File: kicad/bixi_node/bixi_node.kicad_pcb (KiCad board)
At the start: 2 copper layers, 48.3 x 16.5 mm, 8 parts, among them J1 RJ45, P1 CONN_01X03, U1 SP3485CN

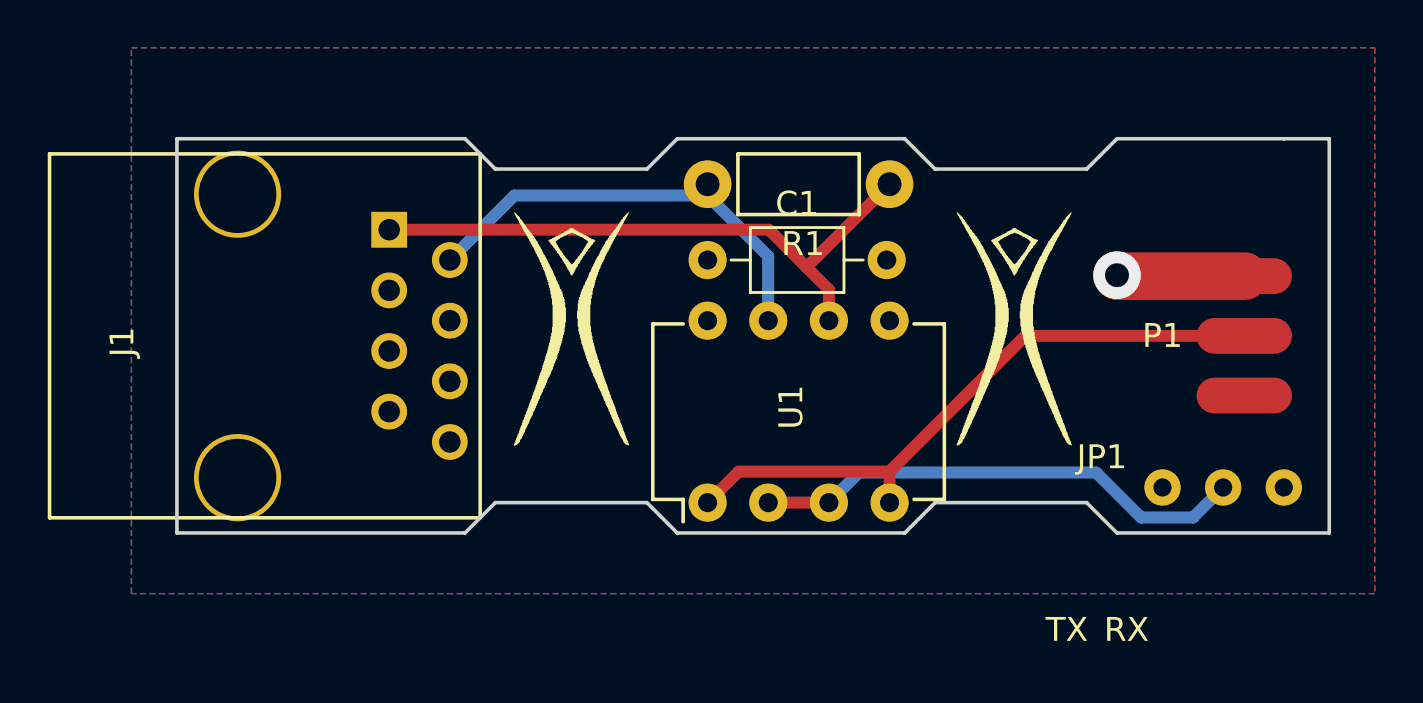
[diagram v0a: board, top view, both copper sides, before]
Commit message: fixes to boards, node still in progress
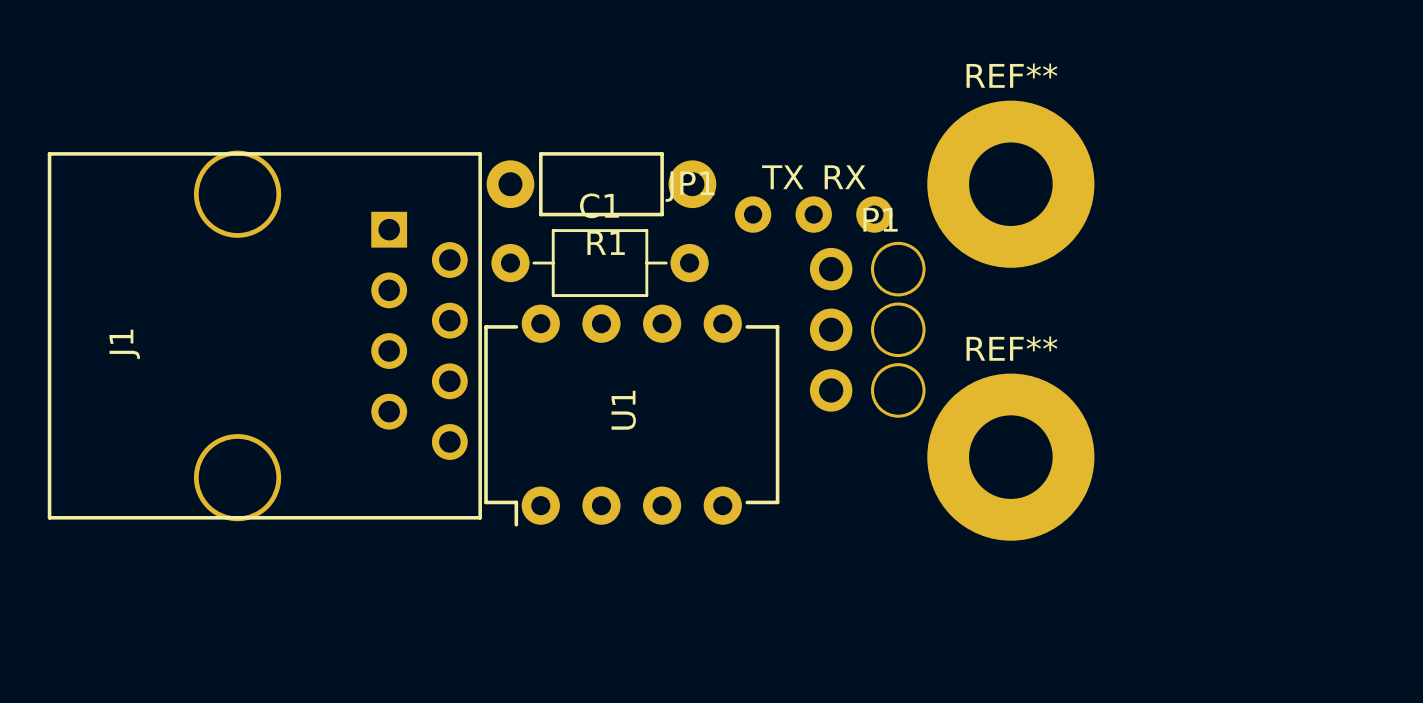
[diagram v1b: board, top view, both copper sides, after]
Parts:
- removed burner-logo1, burner-logo2: , logos:burner-logo-fs
- added REF**: MountingHole_3.5mm_Pad, Mounting_Holes:MountingHole_3.5mm_Pad, F.Cu at (128.9, 85.1)
- added REF**: MountingHole_3.5mm_Pad, Mounting_Holes:MountingHole_3.5mm_Pad, F.Cu at (128.9, 96.5)
- P1: footprint custom:PAD_3X_OVAL_WS2812B -> custom:3-wire-hole-with-relief
- moved JP1 20.6 mm to (120.7, 86.4)
- moved P1 15.2 mm to (123.2, 91.2), turned to 0 degrees
- moved C1 8.26 mm to (108.0, 88.4)
- moved R1 8.25 mm to (108.0, 85.1)
- moved U1 6.99 mm to (109.2, 98.6)
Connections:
- P1 pad 1: VCC -> GND
- P1 pad 3: GND -> Net-(P1-Pad3)
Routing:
- net /DATA: track 26.7 -> 0.00 mm
- net /DATA_DIFF_A: track 25.7 -> 0.00 mm
- net /MODE: track 20.9 -> 0.00 mm
- net /DATA_DIFF_B: track 18.7 -> 0.00 mm
- net GND: track 5.35 -> 0.00 mm, vias 1 -> 0
- removed copper zone on B.Cu, net GND
- removed copper zone on F.Cu, net VCC
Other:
- board outline removed

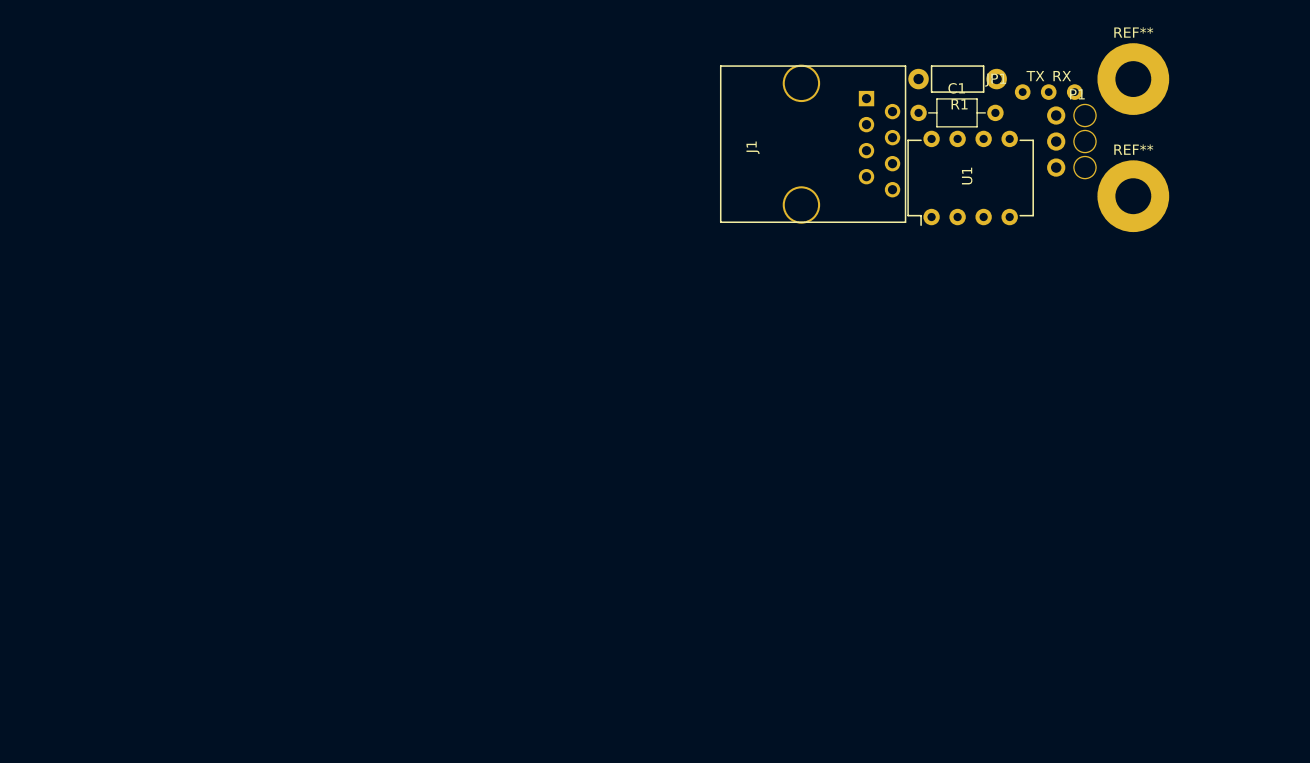
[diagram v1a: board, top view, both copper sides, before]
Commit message: node work for keystone box
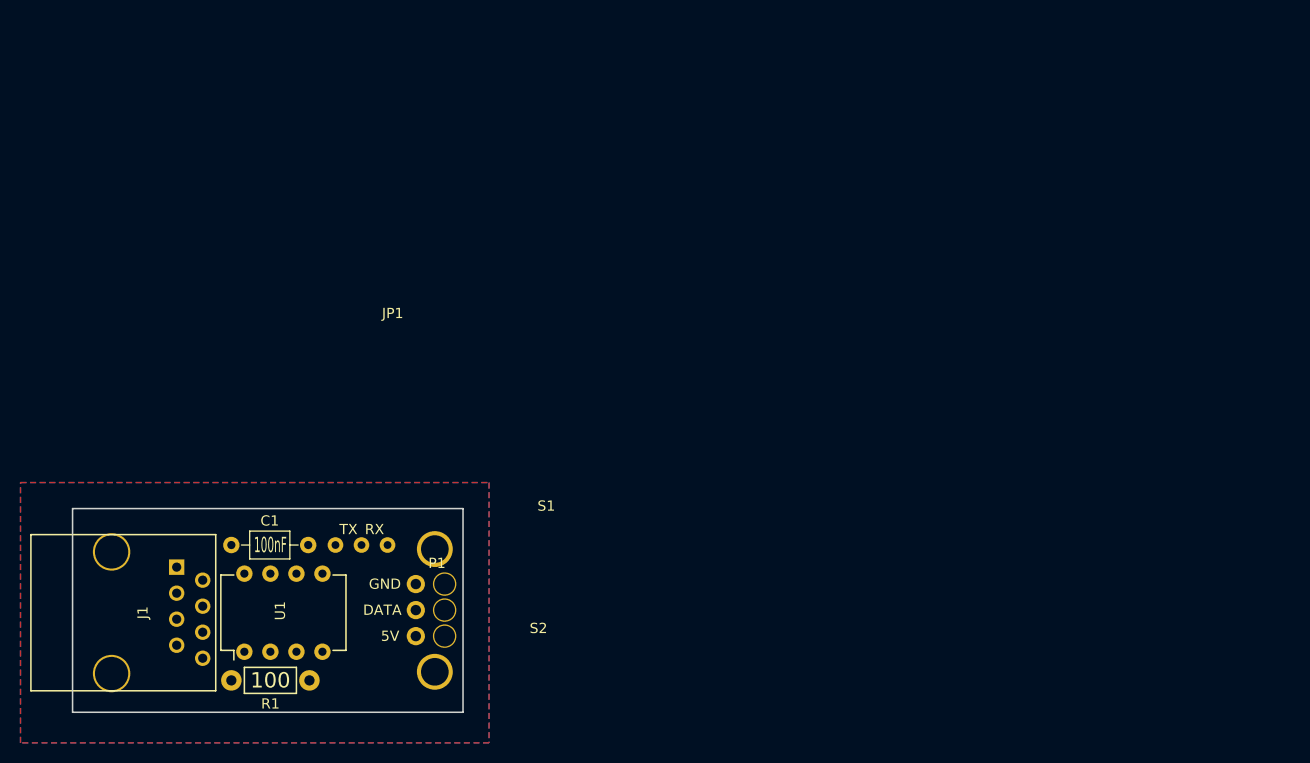
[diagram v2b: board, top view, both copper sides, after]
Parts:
- removed REF** (x2): MountingHole_3.5mm_Pad, Mounting_Holes:MountingHole_3.5mm_Pad
- added S1: MountingHole_2.7mm_Pad, Mounting_Holes:MountingHole_2.7mm_Pad, F.Cu at (60.8, 130.9)
- added S2: MountingHole_2.7mm_Pad, Mounting_Holes:MountingHole_2.7mm_Pad, F.Cu at (60.8, 142.9)
- moved R1 89.1 mm to (40.9, 143.8)
- moved J1 81.4 mm to (29.2, 137.2)
- moved JP1 80.3 mm to (53.6, 130.6)
- moved U1 79.3 mm to (42.2, 141.0)
- moved C1 79.2 mm to (40.9, 130.6)
- moved P1 77.4 mm to (60.7, 136.9)
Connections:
- P1 pad 3: Net-(P1-Pad3) -> VCC
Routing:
- added copper zone on B.Cu, net GND
- added copper zone on F.Cu, net VCC
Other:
- board outline added: 38.1 x 19.9 mm
- net class Default: trace_width 2 -> 0.4; via_dia 2 -> 0.4; via_drill 1 -> 0.3
- board text added: "100"
- board text added: "100nF"
- board text added: "5V"
- board text added: "DATA"
- board text added: "GND"
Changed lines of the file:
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@@
 (kicad_pcb (version 4) (host pcbnew 4.0.6)
   (general
-    (links 15)
-    (no_connects 15)
-    (area 88.370999 79.615 138.819286 102.656762)
+    (links 16)
+    (no_connects 8)
+    (area 20.32 124.46 75.751 149.860001)
     (thickness 1.6)
-    (drawings 2)
+    (drawings 11)
     (tracks 0)
     (zones 0)
     (modules 8)
-    (nets 12)
+    (nets 11)
   )
   (page A4)
@@
   )
   (setup
-    (last_trace_width 2)
+    (last_trace_width 0.4)
     (trace_clearance 0.2)
     (zone_clearance 0.508)
@@
     (segment_width 0.2)
     (edge_width 0.15)
-    (via_size 2)
-    (via_drill 1)
+    (via_size 0.4)
+    (via_drill 0.3)
     (via_min_size 0.4)
     (via_min_drill 0.3)
@@
     (mod_text_size 1 1)
     (mod_text_width 0.15)
-    (pad_size 1.524 1.524)
-    (pad_drill 0.762)
+    (pad_size 3.5 3.5)
+    (pad_drill 2.7)
     (pad_to_mask_clearance 0.2)
     (aux_axis_origin 0 0)
@@
   (net 9 "Net-(J1-Pad5)")
   (net 10 "Net-(J1-Pad6)")
-  (net 11 "Net-(P1-Pad3)")
   (net_class Default "This is the default net class."
     (clearance 0.2)
-    (trace_width 2)
-    (via_dia 2)
-    (via_drill 1)
+    (trace_width 0.4)
+    (via_dia 0.4)
+    (via_drill 0.3)
     (uvia_dia 0.3)
     (uvia_drill 0.1)
@@
     (add_net "Net-(J1-Pad5)")
     (add_net "Net-(J1-Pad6)")
-    (add_net "Net-(P1-Pad3)")
     (add_net VCC)
   )
+  (module Mounting_Holes:MountingHole_2.7mm_Pad locked (layer F.Cu)
+    (at 60.75 142.9255)
+    (descr "Mounting Hole 2.7mm")
+    (tags "mounting hole 2.7mm")
+    (fp_text reference S2 (at 10.116 -4.2415) (layer F.SilkS)
+      (effects (font (size 1 1) (thickness 0.15)))
+    )
+    (fp_text value MountingHole_2.7mm_Pad (at 20.276 5.6645) (layer F.Fab)
+      (effects (font (size 1 1) (thickness 0.15)))
+    )
+    (fp_circle (center 0 0) (end 2.7 0) (layer Cmts.User) (width 0.15))
+    (fp_circle (center 0 0) (end 2.95 0) (layer F.CrtYd) (width 0.05))
+    (pad 1 thru_hole circle (at 0 0) (size 3.5 3.5) (drill 2.7) (layers *.Cu *.Mask))
+  )
   (module Housings_DIP:DIP-8_W7.62mm (layer F.Cu)
-    (at 109.22 98.552 90)
+    (at 42.164 140.97 90)
     (descr "8-lead dip package, row spacing 7.62 mm (300 mils)")
     (tags "dil dip 2.54 300")
@@
   )
   (module Connectors:RJ45_8 (layer F.Cu)
-    (at 96.52 91.44 270)
+    (at 29.21 137.16 270)
     (tags RJ45)
-    (fp_text reference J1 (at 0.254 4.826 270) (layer F.SilkS)
+    (fp_text reference J1 (at 0 -3.048 270) (layer F.SilkS)
       (effects (font (size 1 1) (thickness 0.15)))
     )
@@
   )
   (module Resistors_THT:Resistor_Horizontal_RM7mm (layer F.Cu)
-    (at 107.95 85.09)
+    (at 40.894 143.764)
     (descr "Resistor, Axial,  RM 7.62mm, 1/3W,")
     (tags "Resistor Axial RM 7.62mm 1/3W R3")
-    (fp_text reference R1 (at 4 2.5) (layer F.SilkS)
+    (fp_text reference R1 (at 3.81 2.286) (layer F.SilkS)
       (effects (font (size 1 1) (thickness 0.15)))
     )
@@
   )
   (module custom:jumper_3_pin_fixed (layer F.Cu)
-    (at 120.65 86.36)
-    (fp_text reference JP1 (at -5.08 -1.27) (layer F.SilkS)
-      (effects (font (size 1 1) (thickness 0.15)))
-    )
-    (fp_text value Jumper_NC_Dual (at 0 -0.5) (layer F.Fab)
+    (at 53.594 130.556)
+    (fp_text reference JP1 (at 3.048 -22.606) (layer F.SilkS)
+      (effects (font (size 1 1) (thickness 0.15)))
+    )
+    (fp_text value Jumper_NC_Dual (at 2.794 -19.812) (layer F.Fab)
       (effects (font (size 1 1) (thickness 0.15)))
     )
@@
   )
   (module Capacitors_THT:C_Axial_L3.8mm_D2.6mm_P7.50mm_Horizontal (layer F.Cu)
-    (at 107.95 88.392)
+    (at 40.894 130.556)
     (descr "C, Axial series, Axial, Horizontal, pin pitch=7.5mm, , length*diameter=3.8*2.6mm^2, http://www.vishay.com/docs/45231/arseries.pdf")
     (tags "C Axial series Axial Horizontal pin pitch 7.5mm  length 3.8mm diameter 2.6mm")
@@
   )
   (module custom:3-wire-hole-with-relief (layer F.Cu)
-    (at 123.19 91.186)
+    (at 60.706 136.906)
     (fp_text reference P1 (at 0.254 -4.572) (layer F.SilkS)
       (effects (font (size 1 1) (thickness 0.15)))
     )
-    (fp_text value CONN_01X03 (at -0.27 -0.5) (layer F.Fab)
+    (fp_text value CONN_01X03 (at 23.368 1.27) (layer F.Fab)
       (effects (font (size 1 1) (thickness 0.15)))
     )
@@
       (net 4 /DATA))
     (pad 3 thru_hole circle (at -1.81 2.54) (size 1.778 1.778) (drill 1.016) (layers *.Cu *.Mask)
-      (net 11 "Net-(P1-Pad3)"))
+      (net 1 VCC))
     (pad "" np_thru_hole circle (at 1 -2.54) (size 2.286 2.286) (drill 2.032) (layers *.Cu *.Mask))
     (pad "" np_thru_hole circle (at 1 0) (size 2.286 2.286) (drill 2.032) (layers *.Cu *.Mask))
     (pad "" np_thru_hole circle (at 1 2.54) (size 2.286 2.286) (drill 2.032) (layers *.Cu *.Mask))
   )
-  (module Mounting_Holes:MountingHole_3.5mm_Pad (layer F.Cu)
-    (at 128.905 85.09)
-    (descr "Mounting Hole 3.5mm")
-    (tags "mounting hole 3.5mm")
-    (fp_text reference REF** (at 0 -4.5) (layer F.SilkS)
-      (effects (font (size 1 1) (thickness 0.15)))
-    )
-    (fp_text value MountingHole_3.5mm_Pad (at 0 4.5) (layer F.Fab)
-      (effects (font (size 1 1) (thickness 0.15)))
-    )
-    (fp_circle (center 0 0) (end 3.5 0) (layer Cmts.User) (width 0.15))
-    (fp_circle (center 0 0) (end 3.75 0) (layer F.CrtYd) (width 0.05))
-    (pad 1 thru_hole circle (at 0 0) (size 7 7) (drill 3.5) (layers *.Cu *.Mask))
-  )
-  (module Mounting_Holes:MountingHole_3.5mm_Pad (layer F.Cu)
-    (at 128.905 96.52)
-    (descr "Mounting Hole 3.5mm")
-    (tags "mounting hole 3.5mm")
-    (fp_text reference REF** (at 0 -4.5) (layer F.SilkS)
-      (effects (font (size 1 1) (thickness 0.15)))
-    )
-    (fp_text value MountingHole_3.5mm_Pad (at 0 4.5) (layer F.Fab)
-      (effects (font (size 1 1) (thickness 0.15)))
-    )
-    (fp_circle (center 0 0) (end 3.5 0) (layer Cmts.User) (width 0.15))
-    (fp_circle (center 0 0) (end 3.75 0) (layer F.CrtYd) (width 0.05))
-    (pad 1 thru_hole circle (at 0 0) (size 7 7) (drill 3.5) (layers *.Cu *.Mask))
-  )
-  (gr_text RX (at 121.92 84.836) (layer F.SilkS)
+  (module Mounting_Holes:MountingHole_2.7mm_Pad locked (layer F.Cu)
+    (at 60.75 130.95)
+    (descr "Mounting Hole 2.7mm")
+    (tags "mounting hole 2.7mm")
+    (fp_text reference S1 (at 10.878 -4.204) (layer F.SilkS)
+      (effects (font (size 1 1) (thickness 0.15)))
+    )
+    (fp_text value MountingHole_2.7mm_Pad (at 22.562 -1.41) (layer F.Fab)
+      (effects (font (size 1 1) (thickness 0.15)))
+    )
+    (fp_circle (center 0 0) (end 2.7 0) (layer Cmts.User) (width 0.15))
+    (fp_circle (center 0 0) (end 2.95 0) (layer F.CrtYd) (width 0.05))
+    (pad 1 thru_hole circle (at 0 0) (size 3.5 3.5) (drill 2.7) (layers *.Cu *.Mask))
+  )
+  (gr_text 5V (at 56.388 139.446) (layer F.SilkS)
+    (effects (font (size 1 1) (thickness 0.25)))
+  )
+  (gr_text DATA (at 55.626 136.906) (layer F.SilkS)
+    (effects (font (size 1 1) (thickness 0.25)))
+  )
+  (gr_text GND (at 55.88 134.366) (layer F.SilkS)
+    (effects (font (size 1 1) (thickness 0.25)))
+  )
+  (gr_text 100 (at 44.704 143.764) (layer F.SilkS)
+    (effects (font (size 1.5 1.5) (thickness 0.3)))
+  )
+  (gr_text 100nF (at 44.704 130.556) (layer F.SilkS)
+    (effects (font (size 1.5 0.75) (thickness 0.1875)))
+  )
+  (gr_line (start 25.4 146.8755) (end 63.5 146.8755) (angle 90) (layer Edge.Cuts) (width 0.15))
+  (gr_line (start 63.5 127) (end 63.5 146.8755) (angle 90) (layer Edge.Cuts) (width 0.15))
+  (gr_line (start 25.4 127) (end 25.4 146.8755) (angle 90) (layer Edge.Cuts) (width 0.15))
+  (gr_line (start 25.4 127) (end 63.5 127) (angle 90) (layer Edge.Cuts) (width 0.15))
+  (gr_text RX (at 54.864 129.032) (layer F.SilkS)
     (effects (font (size 1 1) (thickness 0.15)))
   )
-  (gr_text TX (at 119.38 84.836) (layer F.SilkS)
+  (gr_text TX (at 52.324 129.032) (layer F.SilkS)
     (effects (font (size 1 1) (thickness 0.15)))
   )
+  (zone (net 1) (net_name VCC) (layer F.Cu) (hatch edge 0.508)
+    (connect_pads (clearance 0.508))
+    (min_thickness 0.254)
+    (fill yes (arc_segments 16) (thermal_gap 1) (thermal_bridge_width 1))
+    (polygon
+      (pts
+        (xy 66.04 149.86) (xy 20.32 149.86) (xy 20.32 124.46) (xy 66.04 124.46)
+      )
+    )
+  )
+  (zone (net 2) (net_name GND) (layer B.Cu) (hatch edge 0.508)
+    (connect_pads (clearance 0.508))
+    (min_thickness 0.254)
+    (fill yes (arc_segments 16) (thermal_gap 1) (thermal_bridge_width 1))
+    (polygon
+      (pts
+        (xy 66.04 149.86) (xy 20.32 149.86) (xy 20.32 124.46) (xy 66.04 124.46)
+      )
+    )
+  )
 )
